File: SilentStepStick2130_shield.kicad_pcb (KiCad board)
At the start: 4 copper layers, 68.6 x 53.3 mm, 15 parts, among them J1 Conn_01x03, U1 TMC2130_SILENTSTEPSTICK, U2 TMC2130_SILENTSTEPSTICK

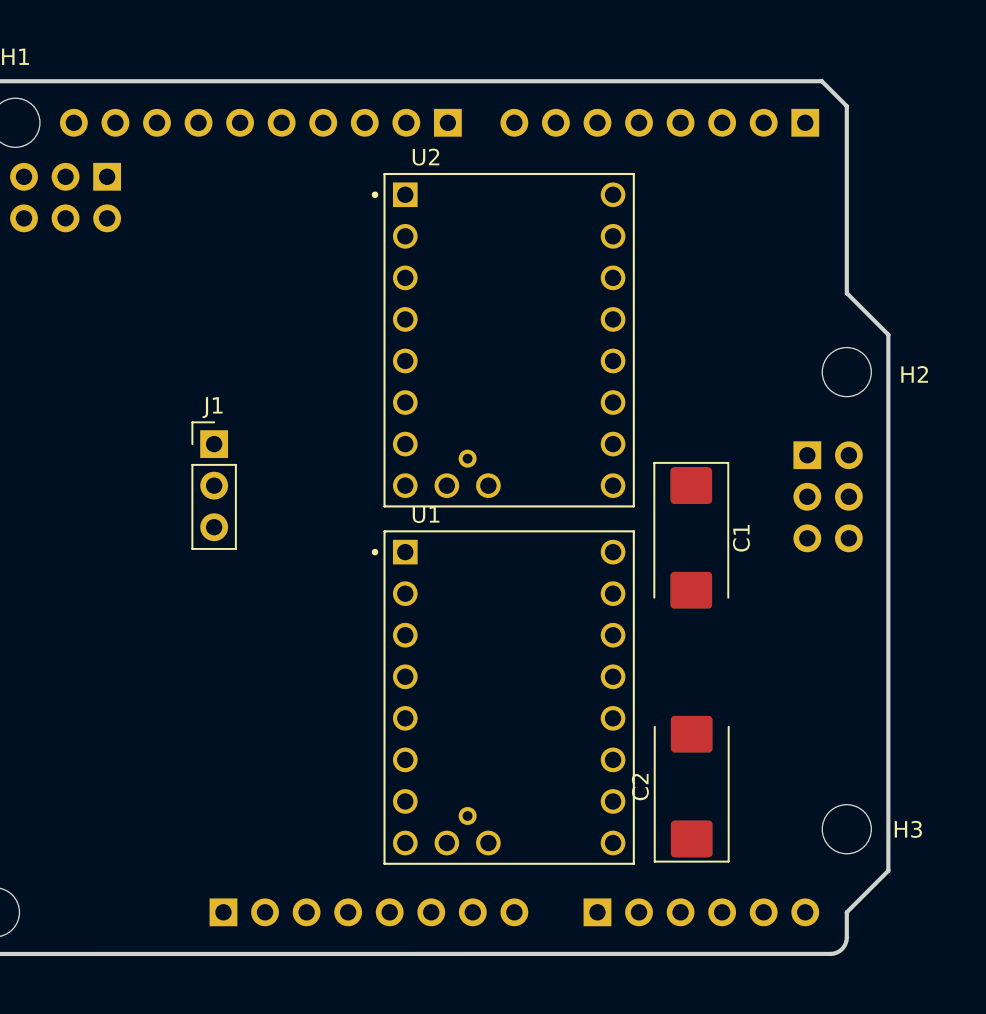
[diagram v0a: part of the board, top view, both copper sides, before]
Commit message: v0
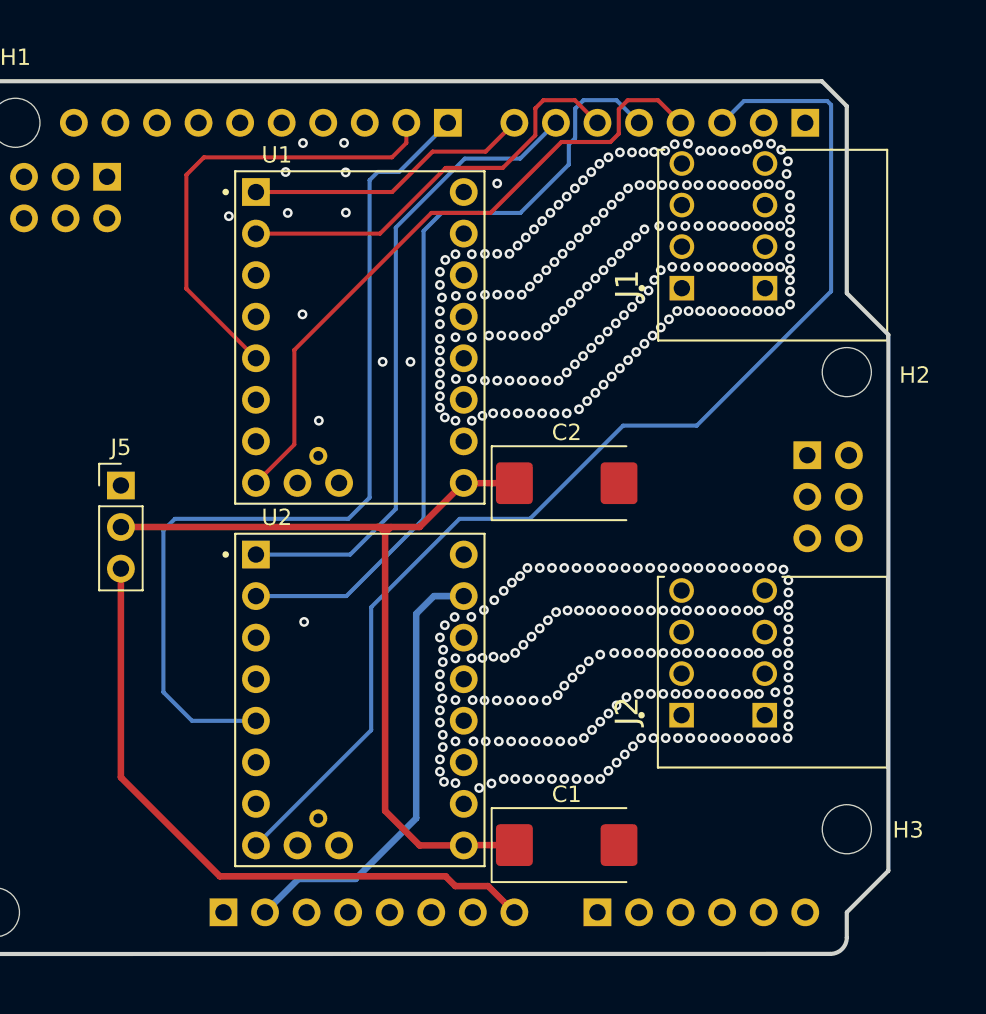
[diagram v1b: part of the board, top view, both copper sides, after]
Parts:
- added J2: Conn_01x04_Socket, LibPersoNadj:CUI_TBL009-254-04BK-2OR, F.Cu at (163.2, 87.7)
- added J5: Conn_01x03, Connector_PinHeader_2.54mm:PinHeader_1x03_P2.54mm_Vertical, F.Cu at (128.9, 73.7)
- J1: value Conn_01x03 -> Conn_01x04_Socket; footprint Connector_PinHeader_2.54mm:PinHeader_1x03_P2.54mm_Vertical -> LibPersoNadj:CUI_TBL009-254-04BK-2OR
- moved J1 30.1 mm to (163.2, 61.6), turned to 90 degrees
- moved U1 23.8 mm to (143.5, 64.6)
- moved U2 23.8 mm to (143.5, 86.8)
- moved C1 20.3 mm to (156.2, 95.6), turned to 0 degrees
- moved C2 20.1 mm to (156.2, 73.5), turned to 0 degrees
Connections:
- C1 pad 1: +5V -> /VM
- C2 pad 1: +5V -> /VM
- IOL1 pad 5: /DIR_2 -> /IO4
- IOL1 pad 6: /DIR_1 -> /IO5
- IOL1 pad 7: /IO6 -> /DIR_2
- IOL1 pad 8: /IO7 -> /DIR_1
- J1 pad 1: +5V -> /OA2_1
- J1 pad 2: +5V -> /OA1_1
- J1 pad 3: /VIN -> /OB1_1
- U1 pad 2: /IO3 -> /IO5
- U1 pad 8: /IO7 -> /IO3
- U1 pad 9: +5V -> /VM
- U2 pad 2: /IO2 -> /IO4
- U2 pad 8: /IO6 -> /IO2
- U2 pad 9: +5V -> /VM
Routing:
- net /IO2: track 0.00 -> 72.3 mm
- net /CS_2: track 0.00 -> 55.4 mm
- net /IOREF: track 0.00 -> 55.0 mm
- net /VM: track 0.00 -> 52.1 mm
- net /SCK: track 0.00 -> 50.9 mm
- net /IO4: track 0.00 -> 48.6 mm
- net /MOSI: track 0.00 -> 47.2 mm
- net +5V: track 0.00 -> 45.9 mm
- net /MISO: track 0.00 -> 42.0 mm
- net /IO3: track 0.00 -> 40.5 mm
- net /VIN: track 0.00 -> 40.2 mm
- net /DIR_2: track 0.00 -> 39.3 mm
- net /CS_1: track 0.00 -> 28.5 mm
- net /IO5: track 0.00 -> 25.8 mm
- net /OB1_1: track 0.00 -> 21.2 mm
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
